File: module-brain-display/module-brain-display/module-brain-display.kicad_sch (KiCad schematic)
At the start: 19 parts, among them J1 Screw_Terminal_01x02, J2 Raspberry_Pi_2_3, J3 Conn_02x20_Top_Bottom, J4 Conn_01x16_Female, T1 Transformer_1P_1S, U1 LCD-016N002L, U2 L7805

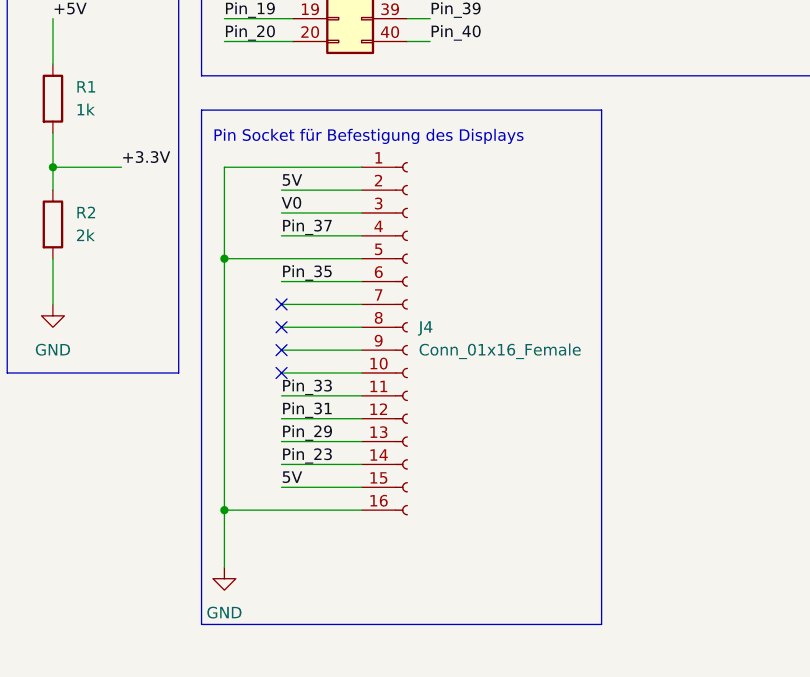
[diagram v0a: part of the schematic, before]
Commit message: Revert "..."
This reverts commit 6093de15b6a411821706cd1d809fe7ad2ca1dc62.
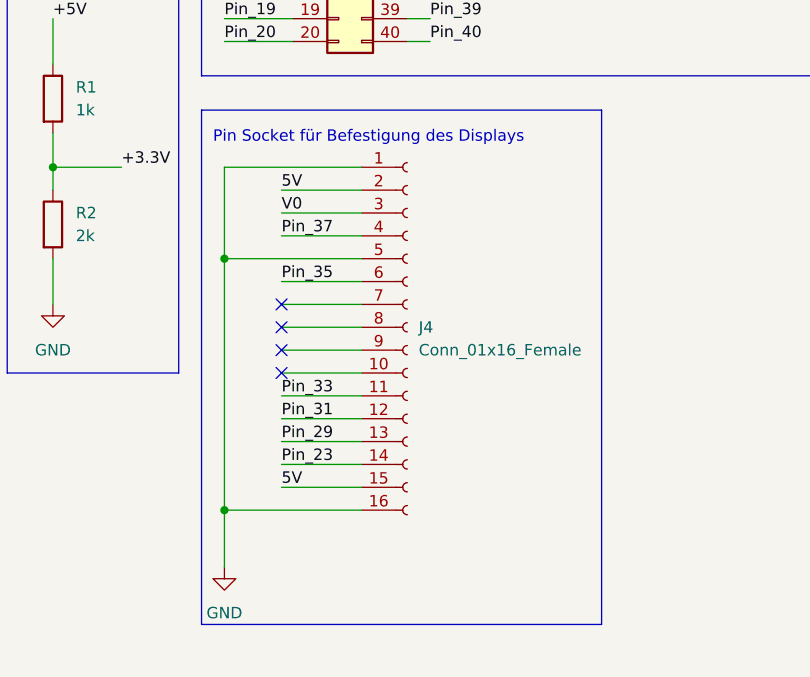
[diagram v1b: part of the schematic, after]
